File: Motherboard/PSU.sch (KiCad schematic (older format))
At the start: 7 parts, among them J4 ATX24, J8 3.3V_HEADER, SW3 SW_SPST_LED, SW4 RESET

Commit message: Large sync
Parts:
- J4: symbol Motherboard-rescue:ATX24-atx24 -> Motherboard-rescue:ATX24-atx24-Motherboard-rescue
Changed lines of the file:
@@
 $Descr A4 11693 8268
 encoding utf-8
-Sheet 6 8
+Sheet 6 10
 Title ""
 Date ""
@@
 $EndDescr
 $Comp
-L Motherboard-rescue:ATX24-atx24 J4
+L Motherboard-rescue:ATX24-atx24-Motherboard-rescue J4
 U 1 1 5C30AAEE
 P 2275 2225

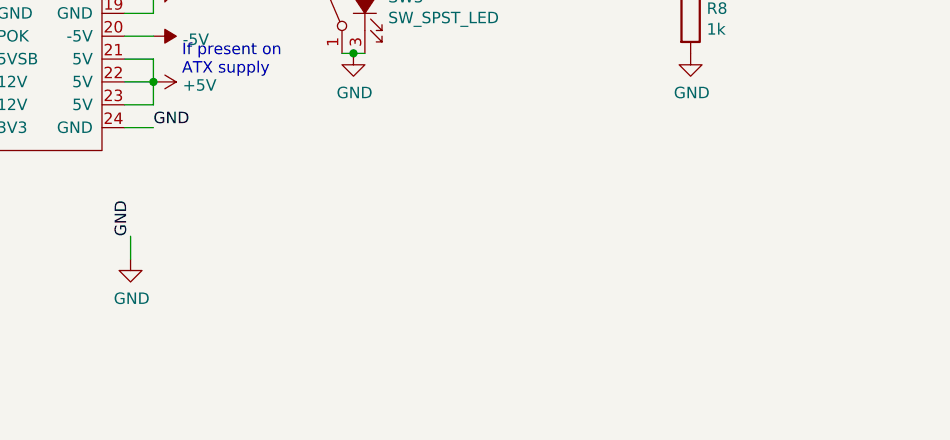
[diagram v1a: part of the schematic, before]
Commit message: LARGE sync
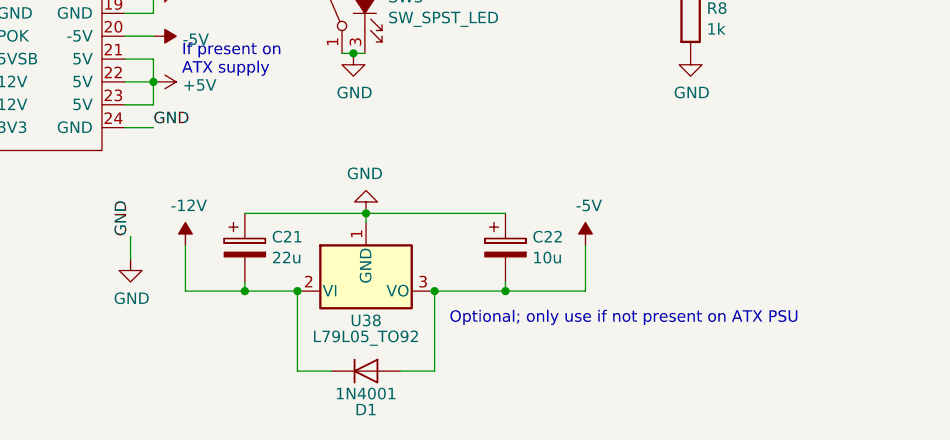
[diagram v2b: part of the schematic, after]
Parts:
- added C21: 22u, Capacitor_THT:CP_Radial_D5.0mm_P2.50mm, symbol Device:CP
- added C22: 10u, Capacitor_THT:CP_Radial_D5.0mm_P2.50mm, symbol Device:CP
- added D1: 1N4001, Diode_THT:D_DO-41_SOD81_P10.16mm_Horizontal, symbol Diode:1N4001
- added U38: L79L05_TO92, Package_TO_SOT_THT:TO-92_Inline, symbol Regulator_Linear:L79L05_TO92
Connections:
- net -12V: now also C21.2, D1.1 (K), U38.2 (VI)
- net -5V: now also C22.2, D1.2 (A), U38.3 (VO)
- net GND: now also C21.1, C22.1, U38.1 (GND)
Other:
- note added: "Optional; only use if not present on ATX PSU"
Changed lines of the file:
@@
 EESchema Schematic File Version 4
 LIBS:Motherboard-cache
-EELAYER 26 0
+EELAYER 29 0
 EELAYER END
 $Descr A4 11693 8268
@@
 $EndComp
 Connection ~ 1150 1150
+$Comp
+L Regulator_Linear:L79L05_TO92 U38
+U 1 1 5C9522CD
+P 3680 3490
+F 0 "U38" H 3680 3360 50  0000 C CNN
+F 1 "L79L05_TO92" H 3680 3290 50  0000 C CNN
+F 2 "Package_TO_SOT_THT:TO-92_Inline" H 3680 3290 50  0001 C CIN
+F 3 "http://www.farnell.com/datasheets/1827870.pdf" H 3680 3490 50  0001 C CNN
+	1    3680 3490
+	1    0    0    -1
+$EndComp
+$Comp
+L Device:CP C21
+U 1 1 5C95256B
+P 3150 3300
+F 0 "C21" H 3268 3346 50  0000 L CNN
+F 1 "22u" H 3268 3255 50  0000 L CNN
+F 2 "Capacitor_THT:CP_Radial_D5.0mm_P2.50mm" H 3188 3150 50  0001 C CNN
+F 3 "~" H 3150 3300 50  0001 C CNN
+	1    3150 3300
+	1    0    0    -1
+$EndComp
+$Comp
+L Device:CP C22
+U 1 1 5C9526F7
+P 4290 3300
+F 0 "C22" H 4408 3346 50  0000 L CNN
+F 1 "10u" H 4408 3255 50  0000 L CNN
+F 2 "Capacitor_THT:CP_Radial_D5.0mm_P2.50mm" H 4328 3150 50  0001 C CNN
+F 3 "~" H 4290 3300 50  0001 C CNN
+	1    4290 3300
+	1    0    0    -1
+$EndComp
+$Comp
+L Diode:1N4001 D1
+U 1 1 5C9527BC
+P 3680 3840
+F 0 "D1" H 3680 3670 50  0000 C CNN
+F 1 "1N4001" H 3680 3740 50  0000 C CNN
+F 2 "Diode_THT:D_DO-41_SOD81_P10.16mm_Horizontal" H 3680 3665 50  0001 C CNN
+F 3 "http://www.vishay.com/docs/88503/1n4001.pdf" H 3680 3840 50  0001 C CNN
+	1    3680 3840
+	1    0    0    -1
+$EndComp
+Wire Wire Line
+	3380 3490 3380 3840
+Wire Wire Line
+	3380 3840 3530 3840
+Wire Wire Line
+	3830 3840 3980 3840
+Wire Wire Line
+	3980 3840 3980 3490
+Wire Wire Line
+	3150 3450 3150 3490
+Wire Wire Line
+	3150 3490 3380 3490
+Connection ~ 3380 3490
+Wire Wire Line
+	3980 3490 4290 3490
+Connection ~ 3980 3490
+Wire Wire Line
+	3150 3150 3680 3150
+Wire Wire Line
+	4290 3450 4290 3490
+Wire Wire Line
+	3680 3190 3680 3150
+Connection ~ 3680 3150
+Wire Wire Line
+	3680 3150 4290 3150
+$Comp
+L power:GND #PWR083
+U 1 1 5C95F2A2
+P 3680 3150
+F 0 "#PWR083" H 3680 2900 50  0001 C CNN
+F 1 "GND" H 3685 2977 50  0000 C CNN
+F 2 "" H 3680 3150 50  0001 C CNN
+F 3 "" H 3680 3150 50  0001 C CNN
+	1    3680 3150
+	-1   0    0    1
+$EndComp
+Wire Wire Line
+	3150 3490 2890 3490
+Wire Wire Line
+	2890 3490 2890 3290
+Connection ~ 3150 3490
+$Comp
+L power:-12V #PWR082
+U 1 1 5C960419
+P 2890 3290
+F 0 "#PWR082" H 2890 3390 50  0001 C CNN
+F 1 "-12V" H 2905 3463 50  0000 C CNN
+F 2 "" H 2890 3290 50  0001 C CNN
+F 3 "" H 2890 3290 50  0001 C CNN
+	1    2890 3290
+	1    0    0    -1
+$EndComp
+Wire Wire Line
+	4640 3490 4640 3290
+$Comp
+L power:-5V #PWR084
+U 1 1 5C961532
+P 4640 3290
+F 0 "#PWR084" H 4640 3390 50  0001 C CNN
+F 1 "-5V" H 4655 3463 50  0000 C CNN
+F 2 "" H 4640 3290 50  0001 C CNN
+F 3 "" H 4640 3290 50  0001 C CNN
+	1    4640 3290
+	1    0    0    -1
+$EndComp
+Wire Wire Line
+	4290 3490 4640 3490
+Connection ~ 4290 3490
+Text Notes 4045 3640 0    50   ~ 0
+Optional; only use if not present on ATX PSU
 $EndSCHEMATC
